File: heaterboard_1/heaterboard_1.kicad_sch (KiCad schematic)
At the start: 12 parts, among them J3 Screw_Terminal_01x06, J4 Conn_02x05_Odd_Even, J7 Screw_Terminal_01x02, U2 TLP175A, U3 TSIC206-TO92

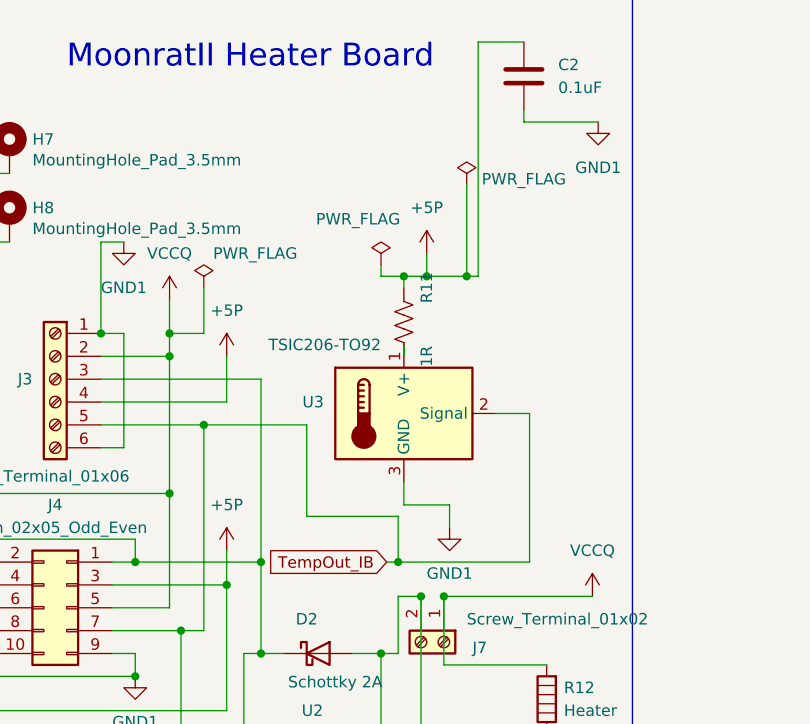
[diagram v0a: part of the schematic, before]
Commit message: heaterboard_1/heaterboard_1.kicad_sch Adding DS18B20 digital thermometer and 4.7 resistor to schematic, add datasheet.
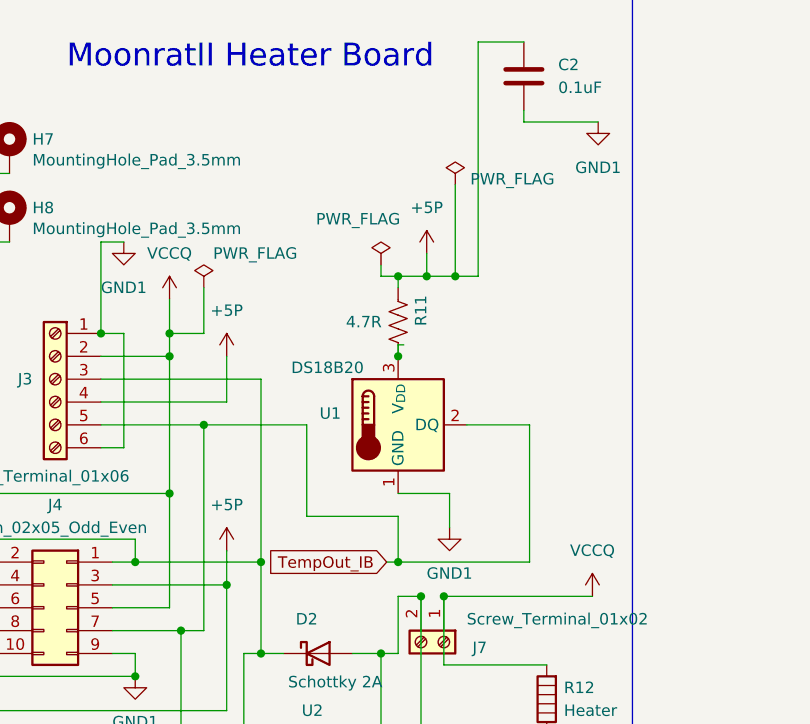
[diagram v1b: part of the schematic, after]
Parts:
- removed U3: TSIC206-TO92, Package_TO_SOT_THT:TO-92_Inline, symbol Sensor_Temperature:TSIC206-TO92
- added U1: DS18B20, Package_TO_SOT_THT:TO-92_Inline, symbol Sensor_Temperature:DS18B20
- R11: value 1R -> 4.7R
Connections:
- net GND1: now also U1.1 (GND)
- net TempOut_IB: now also U1.2 (DQ)
- net at R11.2: now also U1.3 (V_{DD})
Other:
- moved on the sheet: R11
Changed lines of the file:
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@@
   (junction (at 52.07 87.63) (diameter 0) (color 0 0 0 0)
   )
-  (junction (at 76.835 48.26) (diameter 0) (color 0 0 0 0)
-  )
   (junction (at 74.295 90.17) (diameter 0) (color 0 0 0 0)
   )
@@
   (junction (at 43.18 54.61) (diameter 0) (color 0 0 0 0)
   )
+  (junction (at 82.55 48.26) (diameter 0) (color 0 0 0 0)
+  )
   (junction (at 46.99 92.71) (diameter 0) (color 0 0 0 0)
   )
@@
   (junction (at 60.96 90.17) (diameter 0) (color 0 0 0 0)
   )
+  (junction (at 76.2 48.26) (diameter 0) (color 0 0 0 0)
+  )
   (junction (at 50.8 72.39) (diameter 0) (color 0 0 0 0)
   )
-  (junction (at 83.82 48.26) (diameter 0) (color 0 0 0 0)
+  (junction (at 76.2 57.15) (diameter 0) (color 0 0 0 0)
   )
   (junction (at 54.61 64.77) (diameter 0) (color 0 0 0 0)
@@
     (stroke (width 0) (type default))
   )
+  (wire (pts (xy 82.55 48.26) (xy 85.09 48.26))
+    (stroke (width 0) (type default))
+  )
   (wire (pts (xy 81.28 83.82) (xy 81.28 91.44))
     (stroke (width 0) (type default))
   )
+  (wire (pts (xy 76.2 48.26) (xy 74.295 48.26))
+    (stroke (width 0) (type default))
+  )
   (wire (pts (xy 81.28 83.82) (xy 97.79 83.82))
     (stroke (width 0) (type default))
@@
     (stroke (width 0) (type default))
   )
-  (wire (pts (xy 79.375 48.26) (xy 83.82 48.26))
+  (wire (pts (xy 79.375 48.26) (xy 82.55 48.26))
     (stroke (width 0) (type default))
   )
@@
     (stroke (width 0) (type default))
   )
-  (wire (pts (xy 90.805 63.5) (xy 90.805 80.01))
+  (wire (pts (xy 90.805 64.77) (xy 90.805 80.01))
+    (stroke (width 0) (type default))
+  )
+  (wire (pts (xy 76.2 55.88) (xy 76.835 55.88))
     (stroke (width 0) (type default))
   )
@@
     (stroke (width 0) (type default))
   )
-  (wire (pts (xy 85.09 48.26) (xy 83.82 48.26))
-    (stroke (width 0) (type default))
-  )
   (wire (pts (xy 50.8 54.61) (xy 50.8 57.15))
     (stroke (width 0) (type default))
@@
     (stroke (width 0) (type default))
   )
-  (wire (pts (xy 83.82 48.26) (xy 83.82 38.1))
+  (wire (pts (xy 82.55 48.26) (xy 82.55 38.1))
     (stroke (width 0) (type default))
   )
@@
     (stroke (width 0) (type default))
   )
-  (wire (pts (xy 76.835 48.26) (xy 74.295 48.26))
-    (stroke (width 0) (type default))
-  )
   (wire (pts (xy 44.45 87.63) (xy 52.07 87.63))
     (stroke (width 0) (type default))
@@
     (stroke (width 0) (type default))
   )
-  (wire (pts (xy 90.805 63.5) (xy 86.995 63.5))
+  (wire (pts (xy 90.805 64.77) (xy 83.82 64.77))
     (stroke (width 0) (type default))
   )
@@
     (stroke (width 0) (type default))
   )
-  (wire (pts (xy 76.835 48.26) (xy 76.835 49.53))
-    (stroke (width 0) (type default))
-  )
-  (wire (pts (xy 76.835 55.88) (xy 76.835 57.15))
+  (wire (pts (xy 76.2 48.26) (xy 76.2 49.53))
+    (stroke (width 0) (type default))
+  )
+  (wire (pts (xy 76.2 55.88) (xy 76.2 57.15))
     (stroke (width 0) (type default))
   )
@@
     (stroke (width 0) (type default))
   )
-  (wire (pts (xy 81.915 73.66) (xy 76.835 73.66))
+  (wire (pts (xy 81.915 72.39) (xy 76.2 72.39))
     (stroke (width 0) (type default))
   )
@@
     (stroke (width 0) (type default))
   )
-  (wire (pts (xy 76.835 48.26) (xy 79.375 48.26))
-    (stroke (width 0) (type default))
-  )
-  (wire (pts (xy 81.915 73.66) (xy 81.915 76.2))
+  (wire (pts (xy 76.2 48.26) (xy 79.375 48.26))
+    (stroke (width 0) (type default))
+  )
+  (wire (pts (xy 81.915 72.39) (xy 81.915 76.2))
     (stroke (width 0) (type default))
   )
@@
   )
   (wire (pts (xy 76.2 83.82) (xy 78.74 83.82))
-    (stroke (width 0) (type default))
-  )
-  (wire (pts (xy 76.835 73.66) (xy 76.835 71.12))
     (stroke (width 0) (type default))
   )
@@
     )
   )
-  (symbol (lib_id "Device:R_US") (at 76.835 53.34 0) (unit 1)
+  (symbol (lib_id "Device:R_US") (at 76.2 53.34 0) (unit 1)
     (in_bom yes) (on_board yes) (dnp no)
-    (property "Reference" "R11" (at 79.375 49.53 90)
-      (effects (font (size 1.27 1.27)))
-    )
-    (property "Value" "1R" (at 79.375 57.15 90)
-      (effects (font (size 1.27 1.27)))
-    )
-    (property "Footprint" "Resistor_SMD:R_0603_1608Metric_Pad0.98x0.95mm_HandSolder" (at 77.851 53.594 90)
-      (effects (font (size 1.27 1.27)) hide)
-    )
-    (property "Datasheet" "https://www.amazon.com/Momentary-Tactile-Through-Breadboard-Friendly/dp/B07WF76VHT/" (at 76.835 53.34 0)
-      (effects (font (size 1.27 1.27)) hide)
-    )
-    (property "AssemblyType" "SMT" (at 76.835 53.34 0)
-      (effects (font (size 1.27 1.27)) hide)
-    )
-    (property "Cost" "0.0015" (at 76.835 53.34 0)
-      (effects (font (size 1.27 1.27)) hide)
-    )
-    (property "Description" "0.1W ±5% 1Ω 0603 Chip Resistor - Surface Mount ROHS" (at 76.835 53.34 0)
-      (effects (font (size 1.27 1.27)) hide)
-    )
-    (property "Distributor 1" "JLCPCB" (at 76.835 53.34 0)
-      (effects (font (size 1.27 1.27)) hide)
-    )
-    (property "Distributor 1 PN" "C269434" (at 76.835 53.34 0)
-      (effects (font (size 1.27 1.27)) hide)
-    )
-    (property "MPN" "RMC060315%N" (at 76.835 53.34 0)
-      (effects (font (size 1.27 1.27)) hide)
-    )
-    (property "Manufacturer" "TyoHM" (at 76.835 53.34 0)
-      (effects (font (size 1.27 1.27)) hide)
-    )
-    (property "Notes" "" (at 76.835 53.34 0)
+    (property "Reference" "R11" (at 78.74 52.07 90)
+      (effects (font (size 1.27 1.27)))
+    )
+    (property "Value" "4.7R" (at 72.39 53.34 0)
+      (effects (font (size 1.27 1.27)))
+    )
+    (property "Footprint" "Resistor_SMD:R_0603_1608Metric_Pad0.98x0.95mm_HandSolder" (at 77.216 53.594 90)
+      (effects (font (size 1.27 1.27)) hide)
+    )
+    (property "Datasheet" "https://www.amazon.com/Momentary-Tactile-Through-Breadboard-Friendly/dp/B07WF76VHT/" (at 76.2 53.34 0)
+      (effects (font (size 1.27 1.27)) hide)
+    )
+    (property "AssemblyType" "SMT" (at 76.2 53.34 0)
+      (effects (font (size 1.27 1.27)) hide)
+    )
+    (property "Cost" "0.0015" (at 76.2 53.34 0)
+      (effects (font (size 1.27 1.27)) hide)
+    )
+    (property "Description" "0.1W ±5% 1Ω 0603 Chip Resistor - Surface Mount ROHS" (at 76.2 53.34 0)
+      (effects (font (size 1.27 1.27)) hide)
+    )
+    (property "Distributor 1" "JLCPCB" (at 76.2 53.34 0)
+      (effects (font (size 1.27 1.27)) hide)
+    )
+    (property "Distributor 1 PN" "C269434" (at 76.2 53.34 0)
+      (effects (font (size 1.27 1.27)) hide)
+    )
+    (property "MPN" "RMC060315%N" (at 76.2 53.34 0)
+      (effects (font (size 1.27 1.27)) hide)
+    )
+    (property "Manufacturer" "TyoHM" (at 76.2 53.34 0)
+      (effects (font (size 1.27 1.27)) hide)
+    )
+    (property "Notes" "" (at 76.2 53.34 0)
       (effects (font (size 1.27 1.27)) hide)
     )
@@
     )
   )
-  (symbol (lib_id "power:PWR_FLAG") (at 83.82 38.1 0) (unit 1)
+  (symbol (lib_id "power:PWR_FLAG") (at 82.55 38.1 0) (unit 1)
     (in_bom yes) (on_board yes) (dnp no)
-    (property "Reference" "#FLG010" (at 83.82 36.195 0)
-      (effects (font (size 1.27 1.27)) hide)
-    )
-    (property "Value" "PWR_FLAG" (at 90.17 37.465 0)
-      (effects (font (size 1.27 1.27)))
-    )
-    (property "Footprint" "" (at 83.82 38.1 0)
-      (effects (font (size 1.27 1.27)) hide)
-    )
-    (property "Datasheet" "~" (at 83.82 38.1 0)
+    (property "Reference" "#FLG010" (at 82.55 36.195 0)
+      (effects (font (size 1.27 1.27)) hide)
+    )
+    (property "Value" "PWR_FLAG" (at 88.9 37.465 0)
+      (effects (font (size 1.27 1.27)))
+    )
+    (property "Footprint" "" (at 82.55 38.1 0)
+      (effects (font (size 1.27 1.27)) hide)
+    )
+    (property "Datasheet" "~" (at 82.55 38.1 0)
       (effects (font (size 1.27 1.27)) hide)
     )
@@
     )
   )
+  (symbol (lib_id "Sensor_Temperature:DS18B20") (at 76.2 64.77 0) (unit 1)
+    (in_bom yes) (on_board yes) (dnp no)
+    (property "Reference" "U1" (at 69.85 63.5 0)
+      (effects (font (size 1.27 1.27)) (justify right))
+    )
+    (property "Value" "DS18B20" (at 72.39 58.42 0)
+      (effects (font (size 1.27 1.27)) (justify right))
+    )
+    (property "Footprint" "Package_TO_SOT_THT:TO-92_Inline" (at 50.8 71.12 0)
+      (effects (font (size 1.27 1.27)) hide)
+    )
+    (property "Datasheet" "https://cdn-shop.adafruit.com/datasheets/DS18B20.pdf" (at 72.39 58.42 0)
+      (effects (font (size 1.27 1.27)) hide)
+    )
+    (pin "1")
+    (pin "2")
+    (pin "3")
+    (instances
+      (project "heaterboard_1"
+        (path "/9ef5effe-cb46-4a9a-bbbe-a65ab44b9e67"
+          (reference "U1") (unit 1)
+        )
+      )
+    )
+  )
   (symbol (lib_id "power:PWR_FLAG") (at 20.32 40.64 0) (unit 1)
     (in_bom yes) (on_board yes) (dnp no)
@@
         )
       )
-    )
-  )
-  (symbol (lib_id "Sensor_Temperature:TSIC206-TO92") (at 76.835 63.5 0) (unit 1)
-    (in_bom yes) (on_board yes) (dnp no)
-    (property "Reference" "U3" (at 67.945 62.23 0)
-      (effects (font (size 1.27 1.27)) (justify right))
-    )
-    (property "Value" "TSIC206-TO92" (at 74.295 55.88 0)
-      (effects (font (size 1.27 1.27)) (justify right))
-    )
-    (property "Footprint" "Package_TO_SOT_THT:TO-92_Inline" (at 67.945 59.69 0)
-      (effects (font (size 1.27 1.27)) (justify left) hide)
-    )
-    (property "Datasheet" "https://shop.bb-sensors.com/out/media/Datasheet_Digital_Semiconductor_temperatur_sensor_TSIC.pdf" (at 76.835 63.5 0)
-      (effects (font (size 1.27 1.27)) hide)
-    )
-    (property "Description" "Digital temperature sensor, range -50 ... +150 °C, 0.3 K accuracy, TO-92" (at 76.835 63.5 0)
-      (effects (font (size 1.27 1.27)) hide)
-    )
-    (pin "1")
-    (pin "2")
-    (pin "3")
-    (instances
-      (project "heaterboard_1"
-        (path "/9ef5effe-cb46-4a9a-bbbe-a65ab44b9e67"
-          (reference "U3") (unit 1)
-        )
-      )
